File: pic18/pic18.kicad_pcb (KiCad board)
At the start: 2 copper layers, 71.1 x 80.4 mm, 97 parts, among them J1 PORTA, J10 PORTE, J11 5v-3.3v, J12 5v-3.3v, J14 PICKIT3, J15 CONTROL, J2 PORTB, J20 LED'S, J21 BUZZER, J3 Barrel_Jack_Switch, J4 Vin, J5 TECLADO, J6 OLED, J7 PORTD, J8 HC-05, J9 PORTC, SW1 SW_Push, SW2 SW_DIP_x01, U1 PIC18F45K50, U2 3x7Segment, U3 NRF24L01_Breakout, U4 AMS1117-5.0, U5 AMS1117-3.3

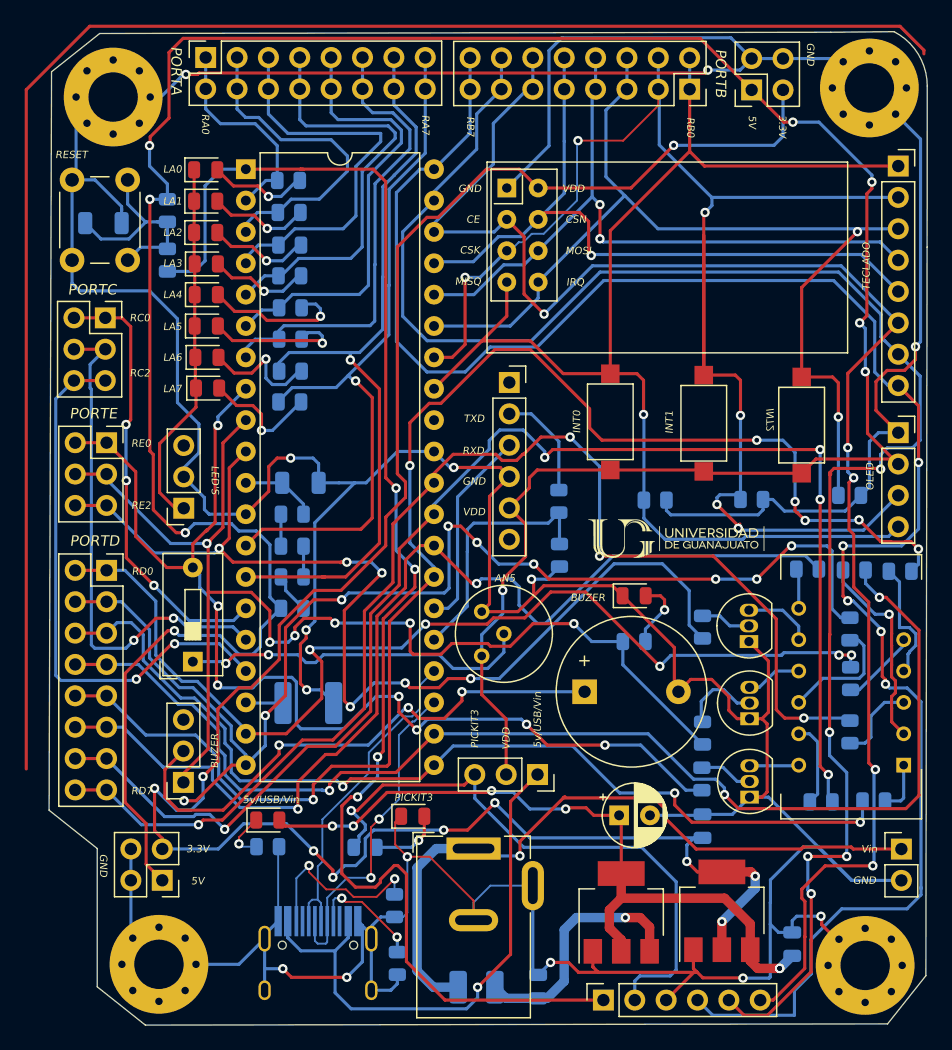
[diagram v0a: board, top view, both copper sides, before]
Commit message: JaPic
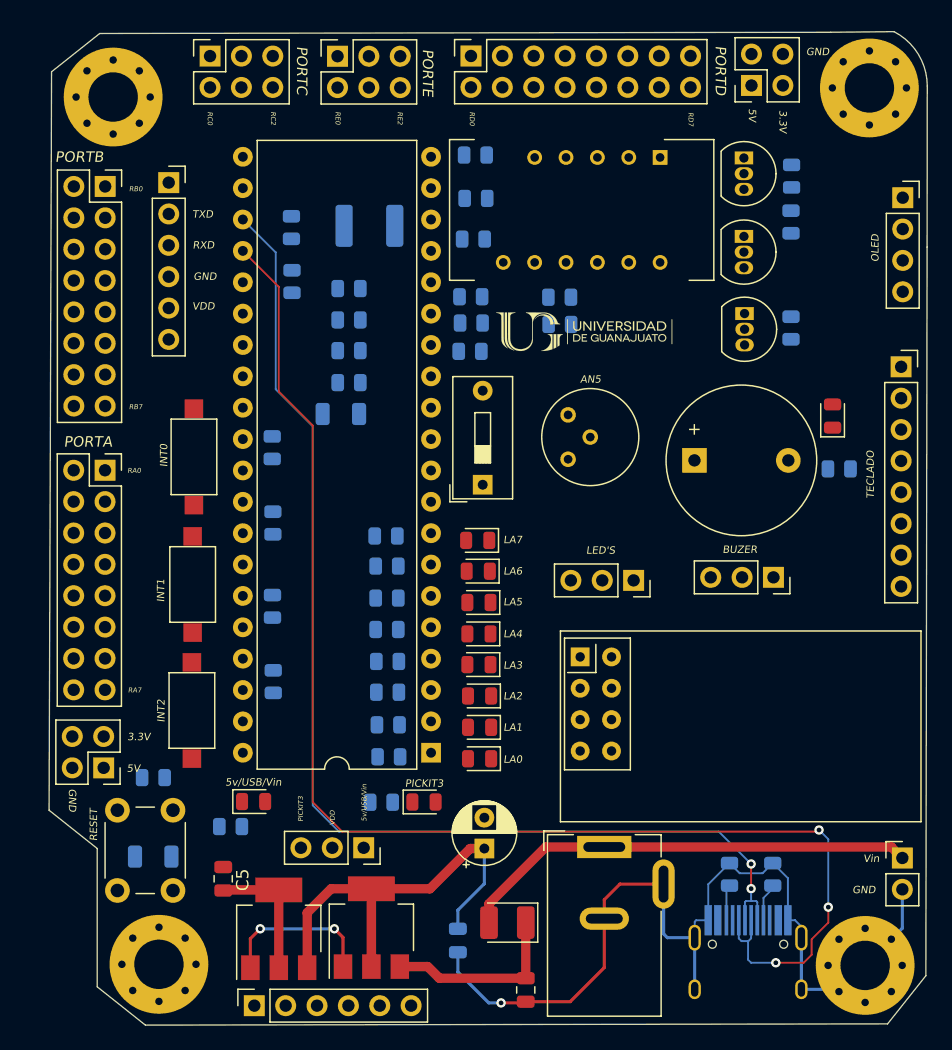
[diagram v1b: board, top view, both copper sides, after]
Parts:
- removed G1: LOGO, FIMEE:japic
- C5, C9, D14: moved to F.Cu
- moved G2 57.7 mm to (47.1, 58.0)
- moved G3 57.7 mm to (46.6, 65.3)
- moved G4 57.7 mm to (46.1, 72.3)
- moved INT2 54.5 mm to (48.5, 74.8)
- moved D11 52.6 mm to (71.8, 78.7), turned to 180 degrees
- moved R29 52.3 mm to (71.0, 41.3)
- moved DIG1 51.8 mm to (93.2, 30.1), turned to 270 degrees
- moved C8 51.5 mm to (45.3, 86.7)
- moved SW1 51.2 mm to (42.4, 89.4)
- moved J7 51.0 mm to (71.1, 21.8), turned to 90 degrees
- moved J21 50.6 mm to (95.6, 64.0), turned to 270 degrees
- moved R32 50.2 mm to (71.3, 36.7), turned to 180 degrees
- moved U1 49.6 mm to (67.8, 78.2), turned to 180 degrees
- moved R24 49.3 mm to (97.0, 31.6), turned to 90 degrees
- moved R31 49.3 mm to (71.5, 33.4), turned to 180 degrees
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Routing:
- net GND: track 481.0 -> 87.1 mm, vias 14 -> 3
- net VDD: track 237.8 -> 0.00 mm, vias 9 -> 0
- net 3.3v: track 170.9 -> 10.8 mm, vias 10 -> 0
- net /RB7: track 153.1 -> 0.00 mm, vias 5 -> 0
- net /RB6: track 141.2 -> 0.00 mm, vias 5 -> 0
- net (no net): track 130.9 -> 0.00 mm
- net /RB5: track 129.8 -> 0.00 mm, vias 5 -> 0
- net /RB1: track 120.7 -> 0.00 mm, vias 6 -> 0
- net /RD4: track 117.8 -> 0.00 mm, vias 7 -> 0
- net /MCLR: track 116.3 -> 0.00 mm, vias 4 -> 0
- net /RD6: track 113.9 -> 0.00 mm, vias 5 -> 0
- net /RB0: track 104.0 -> 0.00 mm, vias 1 -> 0
- net /RD7: track 103.2 -> 0.00 mm, vias 4 -> 0
- net /RD1: track 100.7 -> 0.00 mm, vias 9 -> 0
- net /RD3: track 100.2 -> 0.00 mm, vias 3 -> 0
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
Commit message: JaPic
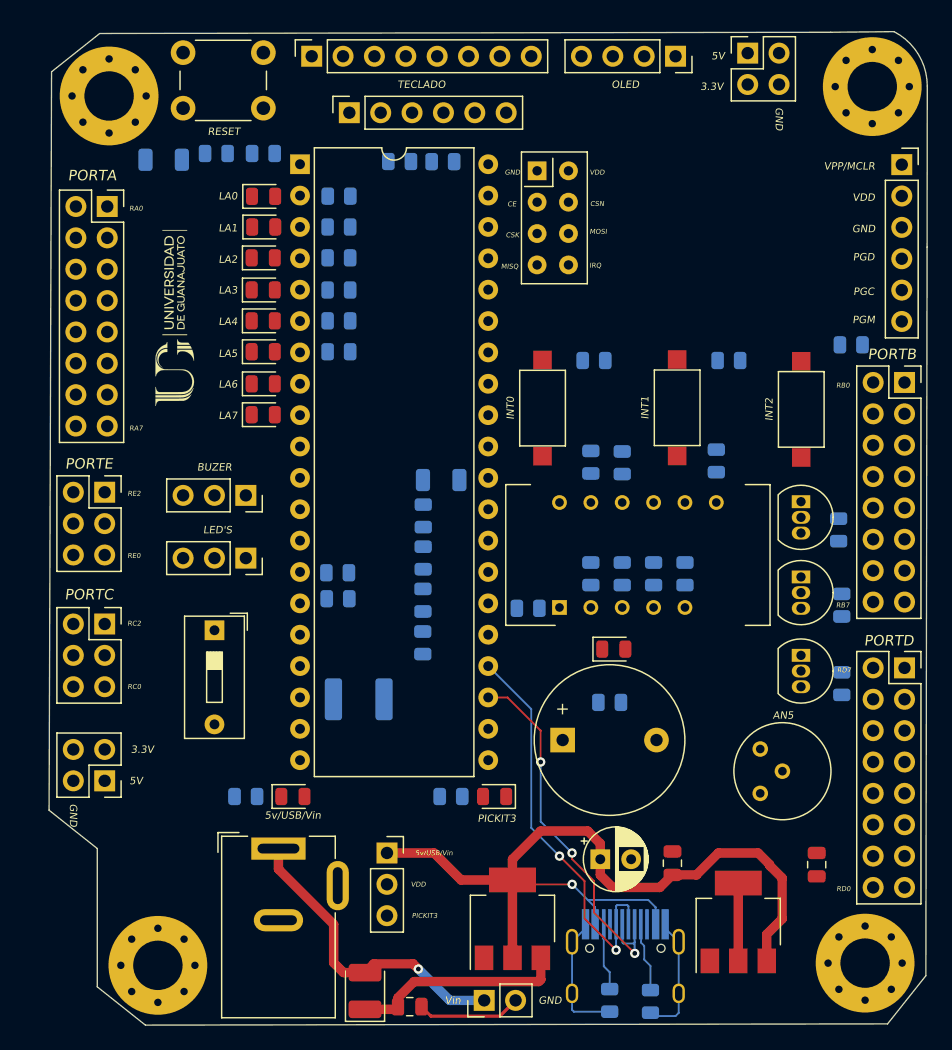
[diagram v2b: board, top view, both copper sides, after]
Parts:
- removed G***: LOGO, FIMEE:usb_logo
- added G1: LOGO, FIMEE:github, B.Cu at (85.6, 35.1)
- C4: moved to F.Cu
- G2: footprint FIMEE:kicad_logo -> FIMEE:open_hardware
- G3: footprint FIMEE:open_hardware -> FIMEE:kicad_logo
- G4: footprint FIMEE:github -> FIMEE:abeja_sf; moved to F.Cu
- G6: footprint FIMEE:abeja_sf -> FIMEE:usb_logo
- moved H2 91.5 mm to (45.7, 95.5)
- moved J14 85.9 mm to (106.0, 30.6), turned to 0 degrees
- moved J11 77.9 mm to (93.5, 21.6), turned to 90 degrees
- moved J12 76.9 mm to (41.4, 80.5), turned to 270 degrees
- moved H4 71.2 mm to (103.6, 24.3)
- moved SW1 68.1 mm to (47.8, 21.6), turned to 0 degrees
- moved J2 66.6 mm to (106.2, 48.3)
- moved G3 60.8 mm to (99.6, 35.6), turned to 180 degrees
- moved J7 60.7 mm to (106.2, 71.4), turned to 0 degrees
- moved G4 58.0 mm to (91.9, 36.7), turned to 0 degrees
- moved H3 57.2 mm to (103.0, 95.3)
- moved C8 56.4 mm to (46.2, 30.2)
- moved INT2 55.0 mm to (97.8, 50.4)
- moved J5 54.0 mm to (58.2, 21.8), turned to 90 degrees
- moved R23 51.4 mm to (101.9, 45.2), turned to 0 degrees
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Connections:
- C4 pad 1: Net-(C3-Pad1) -> 5V
- D1 pad 2: Net-(C3-Pad1) -> 5V
- U4 pad 2: Net-(C3-Pad1) -> 5V
- U5 pad 3: Net-(C3-Pad1) -> 5V
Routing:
- net /RC5: track 111.1 -> 33.4 mm, vias 3 -> 2
- net /RC4: track 94.3 -> 31.5 mm, vias 2 -> 3
- net GND: track 87.1 -> 29.7 mm, vias 3 -> 0
- net 5V: track 0.00 -> 25.3 mm, vias 0 -> 1
- net /Vin: track 37.3 -> 25.1 mm, vias 0 -> 1
- net Net-(C3-Pad1): track 34.6 -> 43.4 mm
- net 3.3v: track 10.8 -> 6.30 mm
- net Net-(R10-Pad2): track 2.91 -> 5.45 mm
- net Net-(R1-Pad2): track 3.12 -> 5.66 mm
- net Net-(C9-Pad1): track 15.1 -> 17.4 mm
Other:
- board text added: "PGM"
- board text removed: "INT0"
- board text removed: "INT1"
- board text removed: "INT2"
